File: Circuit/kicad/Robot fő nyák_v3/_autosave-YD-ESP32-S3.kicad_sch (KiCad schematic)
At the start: 23 parts, among them J14 Conn_02x20_Odd_Even, J15 Conn_02x20_Odd_Even, Q2 bc akármi, Q3 bc akármi, U37 CH343P

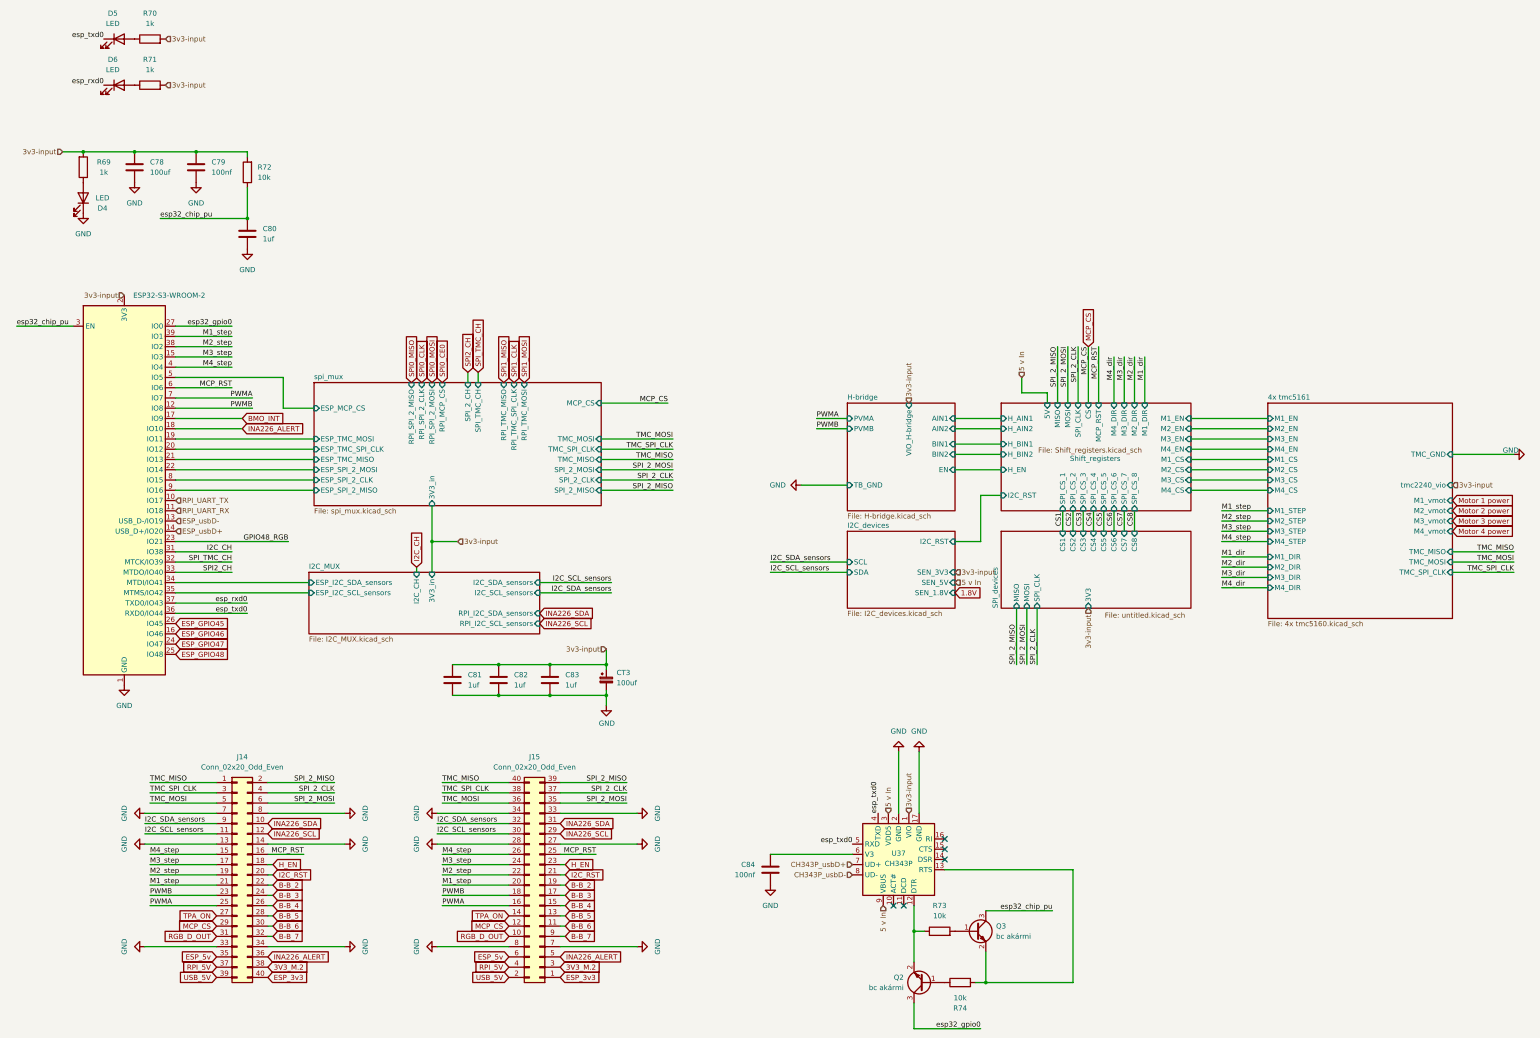
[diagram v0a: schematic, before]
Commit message: updated kicad (big_update)
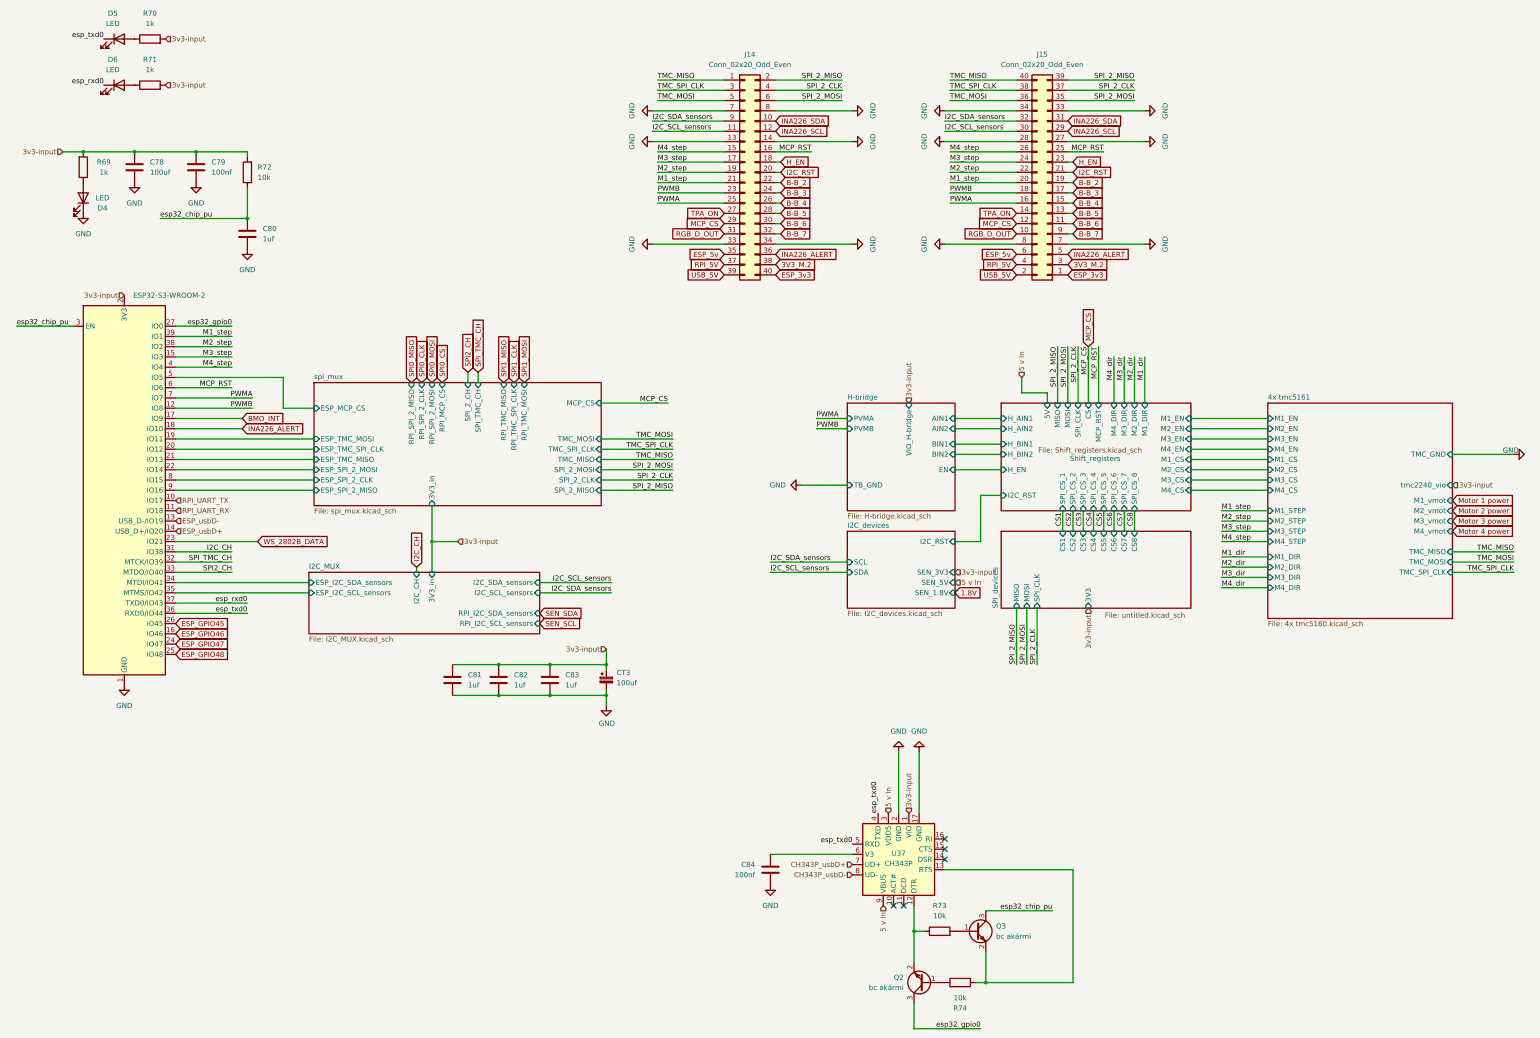
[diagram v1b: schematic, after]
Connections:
- net GPIO48_RGB renamed WS_2802B_DATA
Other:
- moved on the sheet: J14, J15
